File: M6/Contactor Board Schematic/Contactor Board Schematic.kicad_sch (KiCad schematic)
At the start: 12 parts

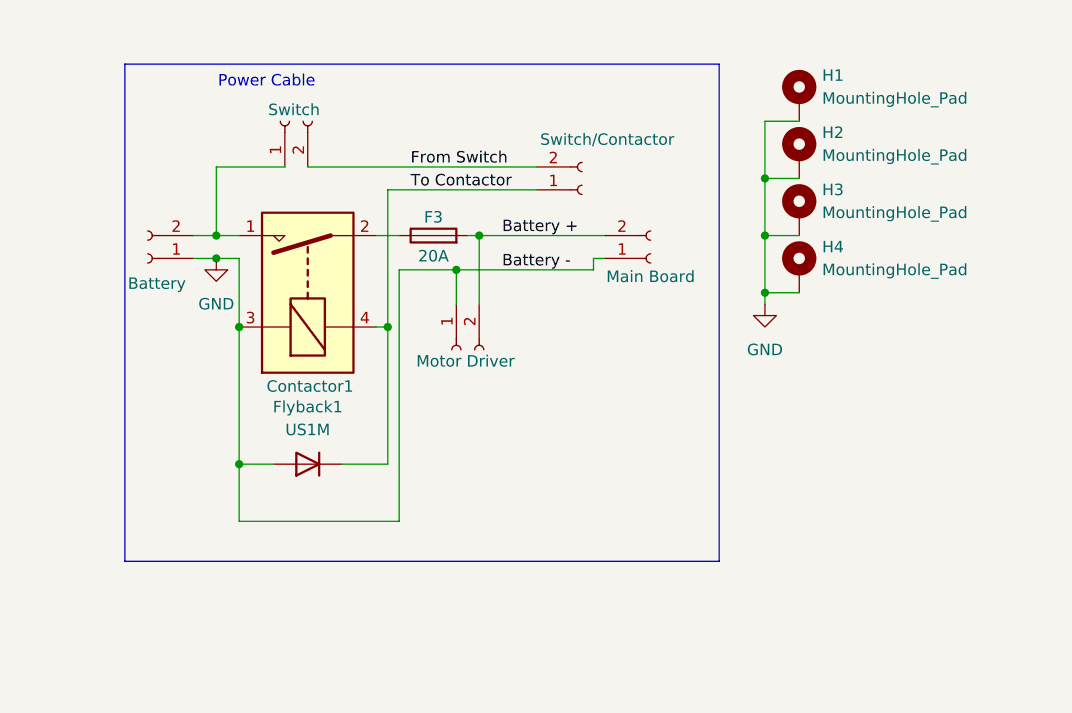
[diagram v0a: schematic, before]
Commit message: CT board progress
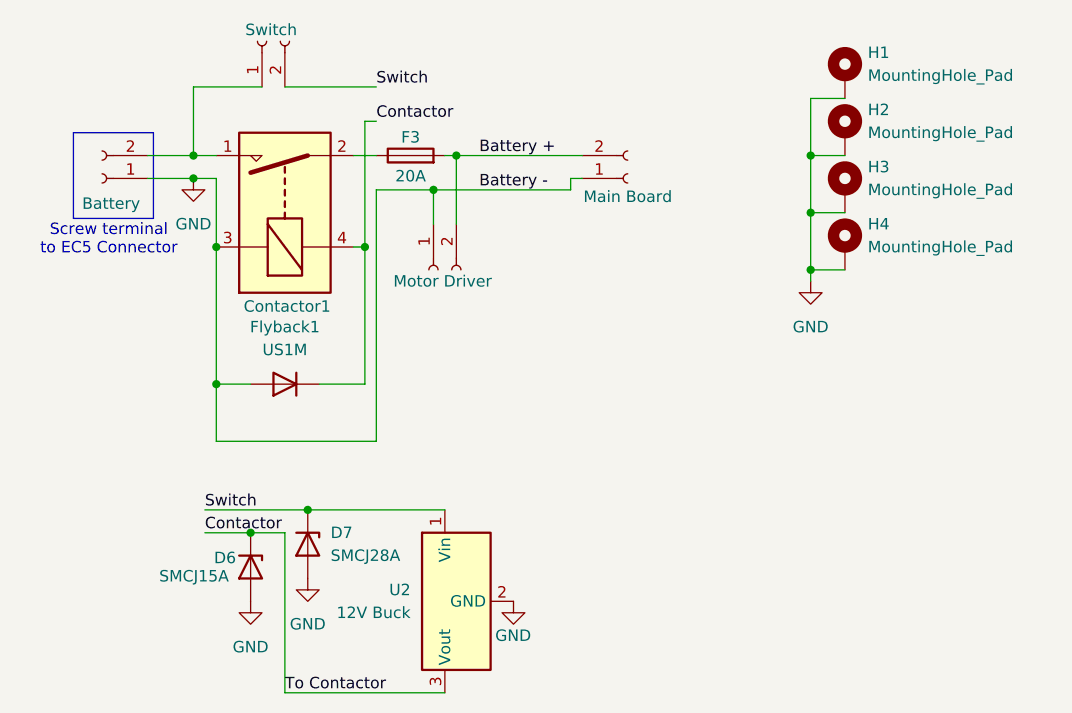
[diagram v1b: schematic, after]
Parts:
- removed J_EXT4: Switch/Contactor, Connector_AMASS:AMASS_XT30PW-F_1x02_P2.50mm_Horizontal, symbol Connector:Conn_01x02_Socket
- added D6: SMCJ15A, Diode_SMD:D_SMC, symbol Device:D_Zener
- added D7: SMCJ28A, Diode_SMD:D_SMC, symbol Device:D_Zener
- added U2: 12V Buck, Converter_DCDC:Converter_DCDC_TRACO_TSR-1_THT, symbol Regulator_Switching:TSR_1-24120
- J_EXT1: footprint Connector_AMASS:AMASS_XT30PW-F_1x02_P2.50mm_Horizontal -> TerminalBlock:TerminalBlock_MaiXu_MX126-5.0-02P_1x02_P5.00mm; digikey (none) -> 277-1667-ND; gobilda 3803-0033-0002 -> (none)
- J_EXT2, J_EXT3, J_EXT5: footprint Connector_AMASS:AMASS_XT30PW-F_1x02_P2.50mm_Horizontal -> Connector_AMASS:AMASS_XT30U-M_1x02_P5.0mm_Vertical
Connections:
- net GND: now also D6.2 (A), D7.2 (A), U2.2 (GND)
- net From Switch renamed Switch
- net Switch: now also D7.1 (K), U2.1 (Vin)
- net To Contactor renamed Contactor
- net Contactor: now also D6.1 (K), U2.3 (Vout)
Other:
- note added: "Screw terminal to EC5 Connector"
- note removed: "Power Cable"
- moved on the sheet: Contactor1, F3, Flyback1, H1, H2, H3, H4
